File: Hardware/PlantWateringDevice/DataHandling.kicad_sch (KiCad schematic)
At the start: 13 parts, among them J1 Conn_02x04_Counter_Clockwise, J5 Conn_02x03_Odd_Even, SW1 SW_DIP_x02, SW3 SW_Push, SW4 SW_DIP_x02, SW7 SW_DIP_x02, U4 PIC10F202-IOT

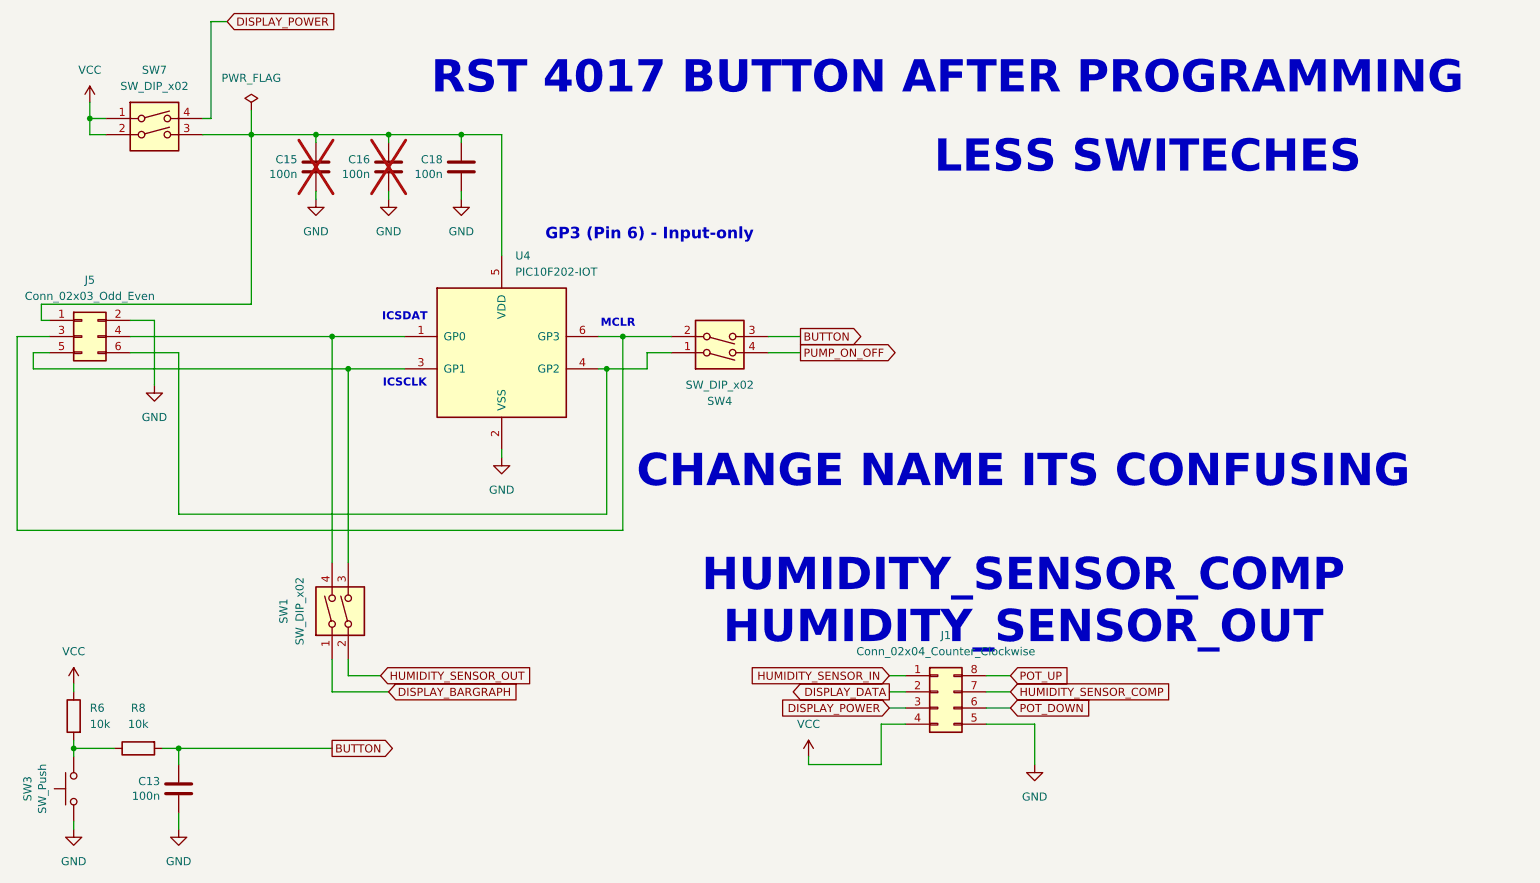
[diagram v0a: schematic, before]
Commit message: fix #29, fix #31
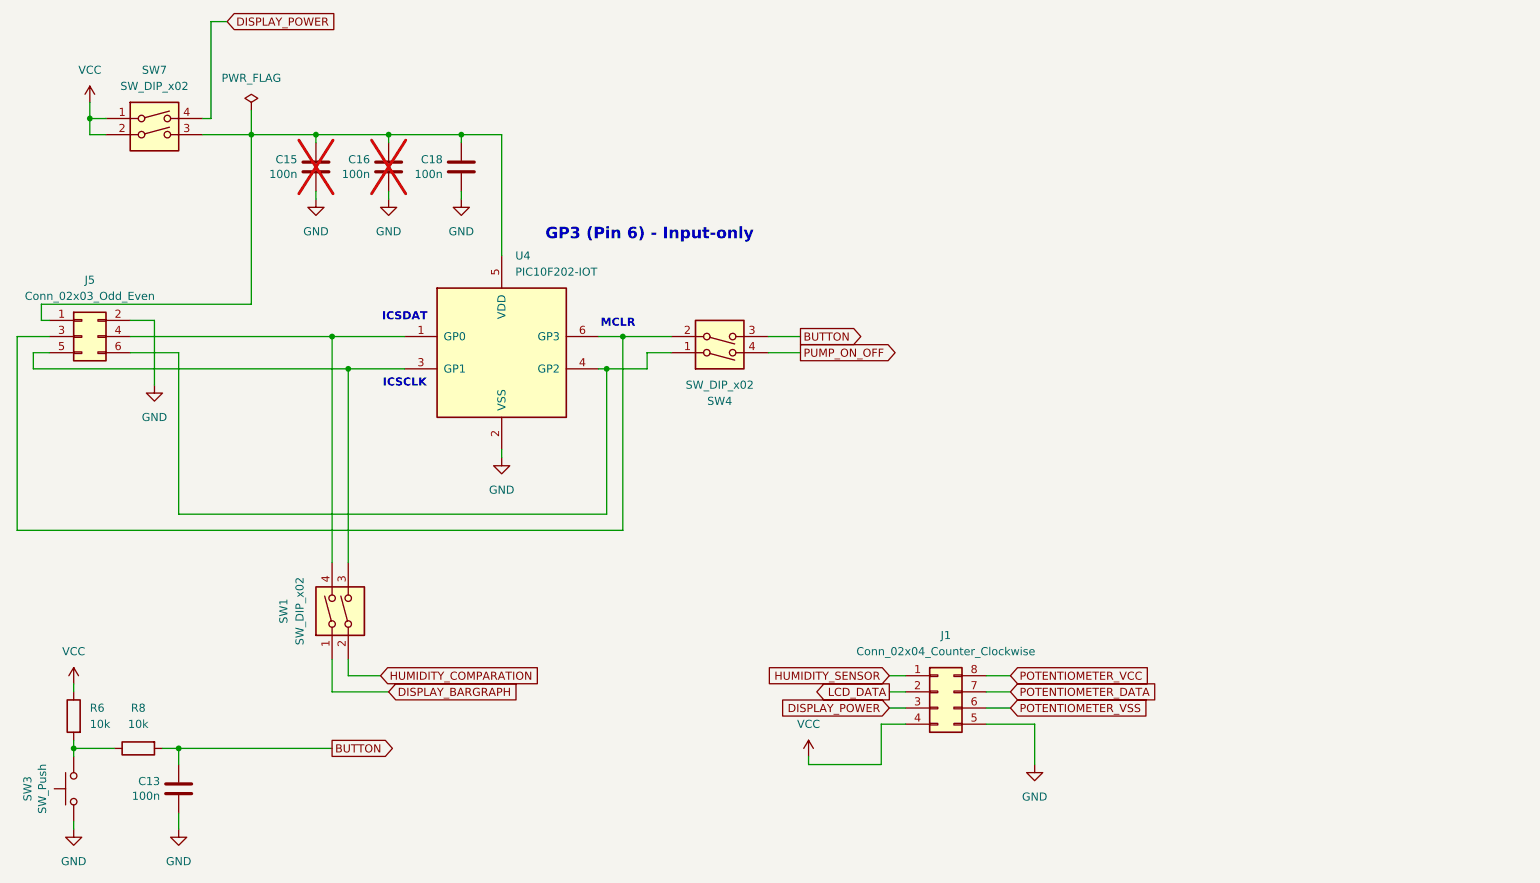
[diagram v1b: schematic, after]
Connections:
- net DISPLAY_DATA renamed LCD_DATA
- net HUMIDITY_SENSOR_COMP renamed POTENTIOMETER_DATA
- net HUMIDITY_SENSOR_IN renamed HUMIDITY_SENSOR
- net HUMIDITY_SENSOR_OUT renamed HUMIDITY_COMPARATION
- net POT_DOWN renamed POTENTIOMETER_VSS
- net POT_UP renamed POTENTIOMETER_VCC
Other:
- note removed: "CHANGE NAME ITS CONFUSING HUMIDITY_SENSOR_COMP HUMIDITY_SENSOR_OUT"
- note removed: "LESS SWITECHES"
- note removed: "RST 4017 BUTTON AFTER PROGRAMMING"
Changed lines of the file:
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@@
-		)
-	)
-	(text "LESS SWITECHES"
-		(exclude_from_sim no)
-		(at 255.27 53.086 0)
-		(effects
-			(font
-				(size 5.08 5.08)
-				(thickness 1.27)
-				(bold yes)
-			)
 		)
 	)
@@
 		)
 	)
-	(text "RST 4017 BUTTON AFTER PROGRAMMING"
-		(exclude_from_sim no)
-		(at 223.774 40.64 0)
-		(effects
-			(font
-				(size 5.08 5.08)
-				(thickness 1.27)
-				(bold yes)
-			)
-		)
-	)
 	(text "MCLR"
 		(exclude_from_sim no)
@@
 				(size 1.27 1.27)
 				(thickness 0.254)
-				(bold yes)
-			)
-		)
-	)
-	(text "CHANGE NAME ITS CONFUSING\n\nHUMIDITY_SENSOR_COMP\nHUMIDITY_SENSOR_OUT"
-		(exclude_from_sim no)
-		(at 235.712 114.808 0)
-		(effects
-			(font
-				(size 5.08 5.08)
-				(thickness 1.27)
 				(bold yes)
 			)
@@
 		)
 	)
-	(global_label "DISPLAY_DATA"
+	(global_label "LCD_DATA"
 		(shape output)
 		(at 214.63 137.16 180)
@@
 		)
 		(property "Intersheetrefs" "${INTERSHEET_REFS}"
-			(at 198.7028 137.16 0)
+			(at 202.6943 137.16 0)
 			(effects
 				(font
@@
 		)
 	)
-	(global_label "POT_DOWN"
+	(global_label "POTENTIOMETER_VSS"
 		(shape input)
 		(at 233.68 139.7 0)
@@
 		)
 		(property "Intersheetrefs" "${INTERSHEET_REFS}"
-			(at 246.5833 139.7 0)
+			(at 256.0779 139.7 0)
 			(effects
 				(font
@@
 		)
 	)
-	(global_label "POT_UP"
+	(global_label "POTENTIOMETER_VCC"
 		(shape input)
 		(at 233.68 134.62 0)
@@
 		)
 		(property "Intersheetrefs" "${INTERSHEET_REFS}"
-			(at 243.8014 134.62 0)
+			(at 256.1989 134.62 0)
 			(effects
 				(font
@@
 		)
 	)
-	(global_label "HUMIDITY_SENSOR_OUT"
+	(global_label "HUMIDITY_COMPARATION"
 		(shape input)
 		(at 134.62 134.62 0)
@@
 		)
 		(property "Intersheetrefs" "${INTERSHEET_REFS}"
-			(at 159.3162 134.62 0)
+			(at 160.2235 134.62 0)
 			(effects
 				(font
@@
 		)
 	)
-	(global_label "HUMIDITY_SENSOR_IN"
+	(global_label "HUMIDITY_SENSOR"
 		(shape input)
 		(at 214.63 134.62 180)
@@
 		)
 		(property "Intersheetrefs" "${INTERSHEET_REFS}"
-			(at 191.6271 134.62 0)
+			(at 194.53 134.62 0)
 			(effects
 				(font
@@
 		)
 	)
-	(global_label "HUMIDITY_SENSOR_COMP"
+	(global_label "POTENTIOMETER_DATA"
 		(shape input)
 		(at 233.68 137.16 0)
@@
 		)
 		(property "Intersheetrefs" "${INTERSHEET_REFS}"
-			(at 260.0695 137.16 0)
-			(effects
-				(font
+			(at 256.9851 137.16 0)
+			(effects
+				(font
